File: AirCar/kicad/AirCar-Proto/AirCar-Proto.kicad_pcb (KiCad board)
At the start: 2 copper layers, 76.2 x 55.9 mm, 22 parts, among them J1 Conn_01x05, J2 Conn_01x20_Socket, J3 Conn_01x06, J4 PJ-102A, J5 Conn_01x20_Socket, SW2 SW_SPDT, U1 Pico, U2 LDL212PU50R, U3 TXU0104BQAR

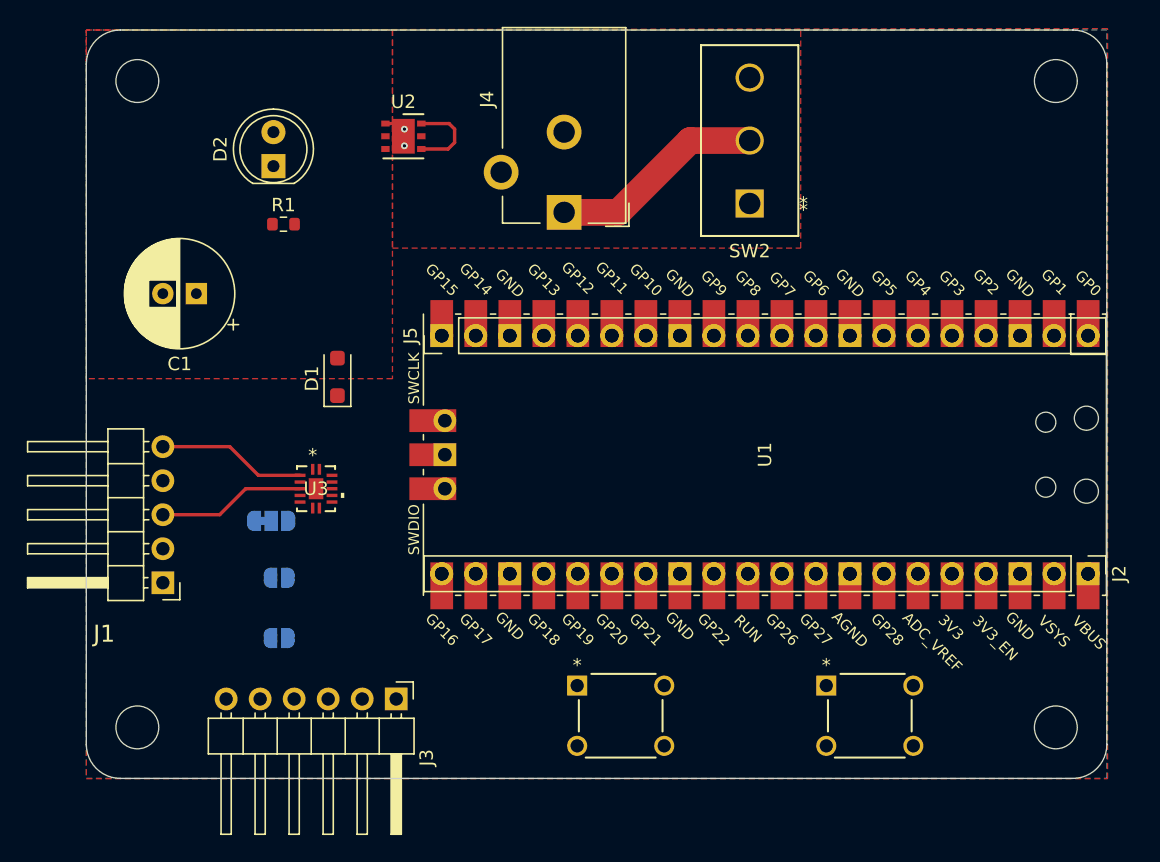
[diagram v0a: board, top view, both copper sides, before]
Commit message: possible rev 0.1 candidate
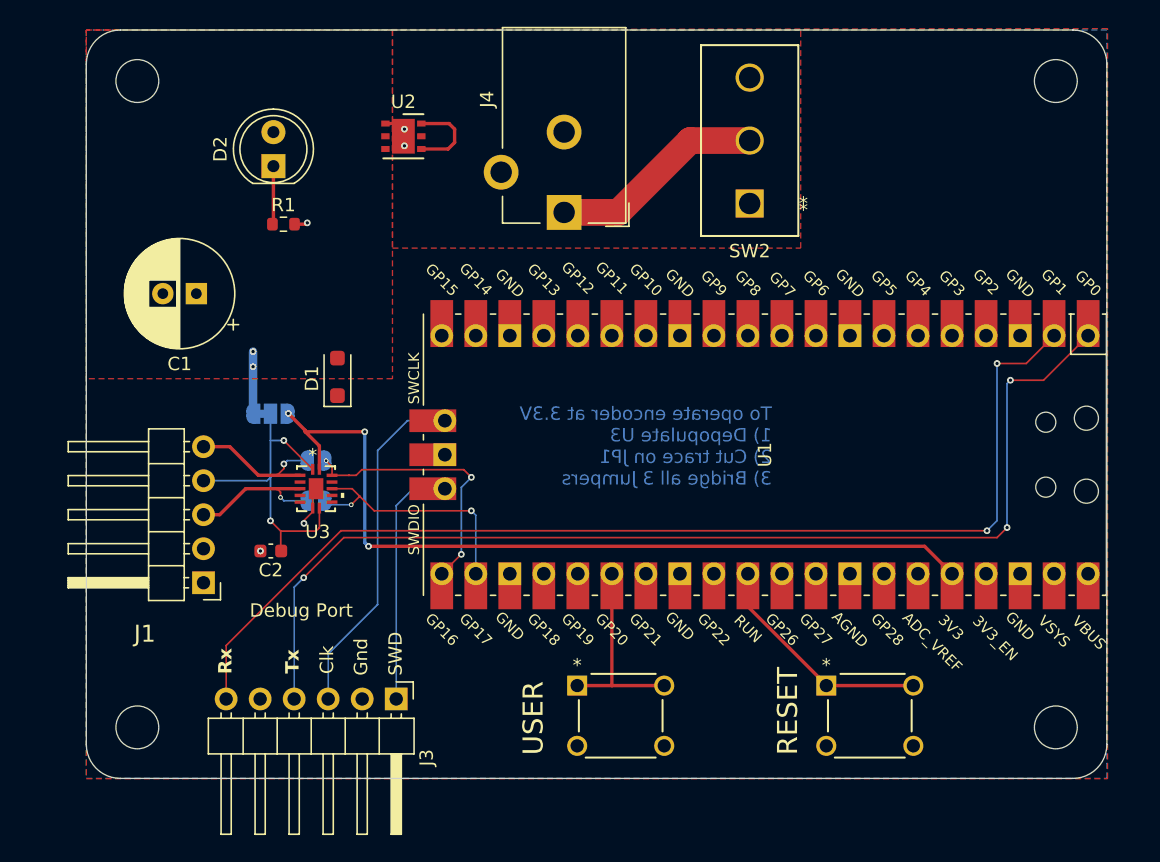
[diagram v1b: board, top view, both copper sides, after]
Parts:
- removed J2, J5: Conn_01x20_Socket, Connector_PinHeader_2.54mm:PinHeader_1x20_P2.54mm_Vertical
- added C2: 0.1uF, Capacitor_SMD:C_0603_1608Metric, F.Cu at (77.3, 140.5)
- moved JP3 10.6 mm to (80.7, 136.8)
- moved JP2 9.17 mm to (80.7, 133.8)
- moved JP1 8.00 mm to (77.2, 130.2)
- moved J1 3.03 mm to (72.2, 142.9)
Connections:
- U1 pad 10: Net-(J5-Pin_11) -> unconnected-(U1-GPIO7-Pad10)
- U1 pad 11: Net-(J5-Pin_10) -> unconnected-(U1-GPIO8-Pad11)
- U1 pad 12: Net-(J5-Pin_9) -> unconnected-(U1-GPIO9-Pad12)
- U1 pad 14: Net-(J5-Pin_7) -> unconnected-(U1-GPIO10-Pad14)
- U1 pad 15: Net-(J5-Pin_6) -> unconnected-(U1-GPIO11-Pad15)
- U1 pad 16: Net-(J5-Pin_5) -> unconnected-(U1-GPIO12-Pad16)
- U1 pad 17: Net-(J5-Pin_4) -> unconnected-(U1-GPIO13-Pad17)
- U1 pad 19: Net-(J5-Pin_2) -> unconnected-(U1-GPIO14-Pad19)
- U1 pad 20: Net-(J5-Pin_1) -> unconnected-(U1-GPIO15-Pad20)
- U1 pad 24: Net-(J2-Pin_17) -> unconnected-(U1-GPIO18-Pad24)
- U1 pad 25: Net-(J2-Pin_16) -> unconnected-(U1-GPIO19-Pad25)
- U1 pad 27: Net-(J2-Pin_14) -> unconnected-(U1-GPIO21-Pad27)
- U1 pad 29: Net-(J2-Pin_12) -> unconnected-(U1-GPIO22-Pad29)
- U1 pad 31: Net-(J2-Pin_10) -> unconnected-(U1-GPIO26_ADC0-Pad31)
- U1 pad 32: Net-(J2-Pin_9) -> unconnected-(U1-GPIO27_ADC1-Pad32)
- U1 pad 34: Net-(J2-Pin_7) -> unconnected-(U1-GPIO28_ADC2-Pad34)
- U1 pad 35: Net-(J2-Pin_6) -> unconnected-(U1-ADC_VREF-Pad35)
- U1 pad 37: Net-(J2-Pin_4) -> unconnected-(U1-3V3_EN-Pad37)
- U1 pad 4: Net-(J5-Pin_17) -> unconnected-(U1-GPIO2-Pad4)
- U1 pad 40: Net-(J2-Pin_1) -> unconnected-(U1-VBUS-Pad40)
- U1 pad 5: Net-(J5-Pin_16) -> unconnected-(U1-GPIO3-Pad5)
- U1 pad 6: Net-(J5-Pin_15) -> unconnected-(U1-GPIO4-Pad6)
- U1 pad 7: Net-(J5-Pin_14) -> unconnected-(U1-GPIO5-Pad7)
- U1 pad 9: Net-(J5-Pin_12) -> unconnected-(U1-GPIO6-Pad9)
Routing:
- net /PicoRx: track 0.00 -> 82.3 mm, vias 0 -> 2
- net /PicoTx: track 0.00 -> 81.7 mm, vias 0 -> 3
- net /V3P3: track 0.00 -> 62.7 mm, vias 0 -> 3
- net Net-(J3-Pin_3): track 0.00 -> 26.0 mm
- net /Venc: track 0.00 -> 24.2 mm, vias 0 -> 2
- net /Lag_3P3: track 0.00 -> 20.2 mm, vias 0 -> 3
- net /Lead_3P3: track 0.00 -> 18.9 mm, vias 0 -> 2
- net Net-(J3-Pin_1): track 0.00 -> 18.6 mm
- net Net-(U1-RUN): track 0.00 -> 17.2 mm
- net Net-(U1-GPIO20): track 0.00 -> 14.9 mm
- net /V5p0: track 0.00 -> 4.64 mm, vias 0 -> 2
- net Net-(D2-K): track 0.00 -> 4.37 mm
- net GND: track 2.92 -> 6.88 mm, vias 2 -> 5
- net /Lead: track 11.0 -> 10.9 mm, vias 0 -> 1
- net /Lag: track 11.1 -> 11.0 mm, vias 0 -> 1
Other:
- board text added: "Clk"
- board text added: "Debug Port"
- board text added: "Gnd"
- board text added: "RESET"
- board text added: "Rx"
- board text added: "SWD"
- board text added: "To operate encoder at 3.3V 1) Depopulate U3 2) Cut trace on JP1 3) Bridge all 3 Jumpers"
- board text added: "Tx"
- board text added: "USER"
